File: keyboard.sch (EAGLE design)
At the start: 11 parts

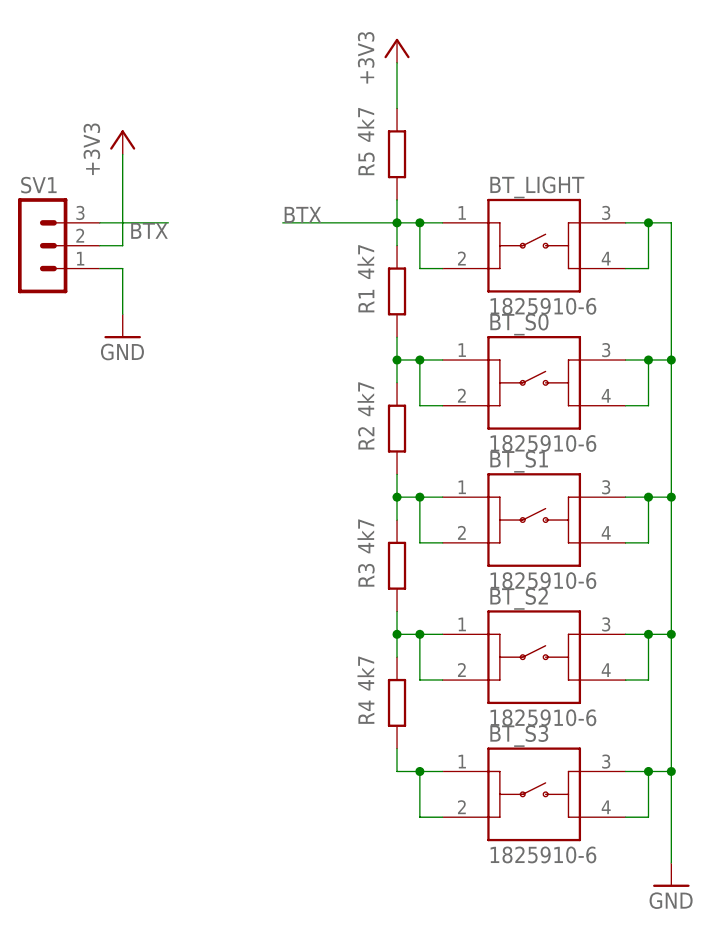
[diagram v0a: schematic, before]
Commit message: upd
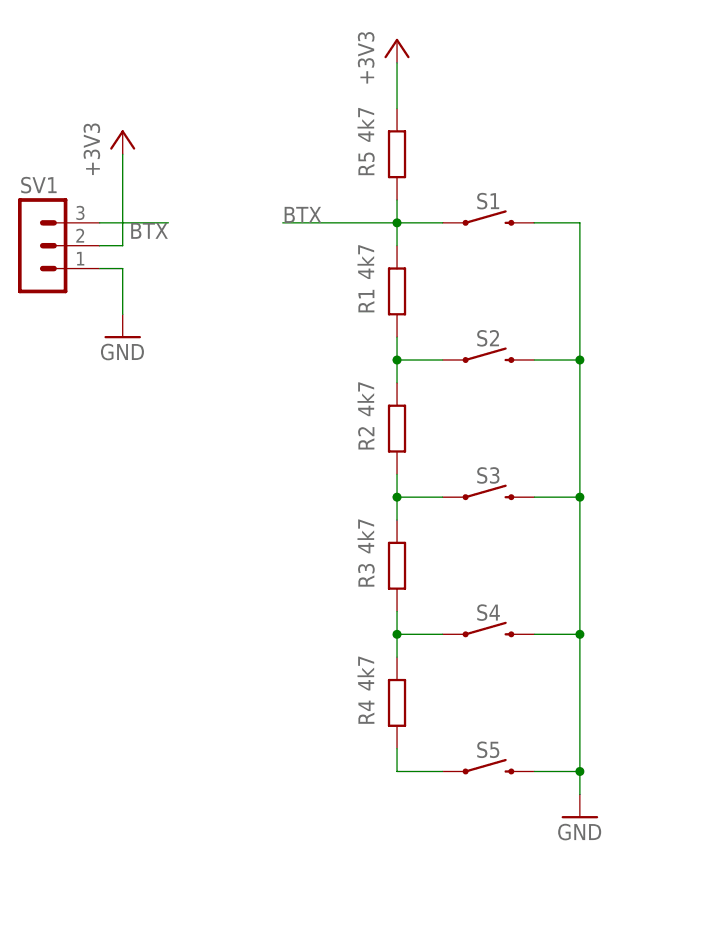
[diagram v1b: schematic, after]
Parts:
- removed BT_LIGHT, BT_S0, BT_S1, BT_S2, BT_S3: 1825910-6, Switch:1825910-6
- added S1, S2, S3, S4, S5: MOMENTARY-SWITCH-SPST-PTH-6.0MM, SparkFun-Switches:MOMENTARY-SWITCH-SPST-PTH-6.0MM
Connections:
- net BTX: now also S1.1; no longer BT_LIGHT.1, BT_LIGHT.2
- net GND: now also S1.2, S2.2, S3.2, S4.2, S5.2; no longer BT_LIGHT.3, BT_LIGHT.4, BT_S0.3, BT_S0.4, BT_S1.3, BT_S1.4, BT_S2.3, BT_S2.4, BT_S3.3, BT_S3.4
- net N$2: now also S4.1; no longer BT_S2.1, BT_S2.2
- net N$3: now also S5.1; no longer BT_S3.1, BT_S3.2
- net N$5: now also S3.1; no longer BT_S1.1, BT_S1.2
- net N$6: now also S2.1; no longer BT_S0.1, BT_S0.2
